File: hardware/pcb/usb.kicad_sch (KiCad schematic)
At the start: 6 parts, among them J3 USB_C_Receptacle_USB2.0_16P, U5 ECMF02-2AMX6

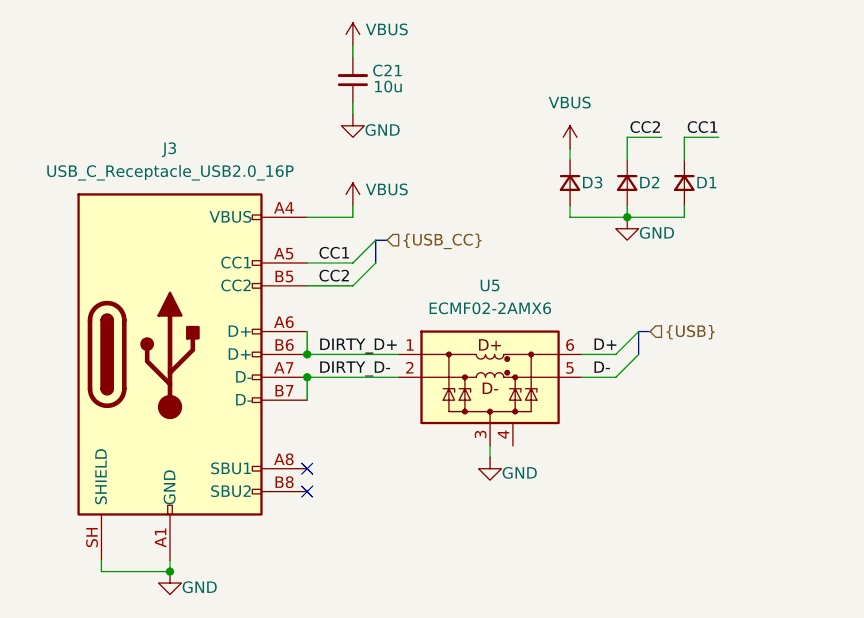
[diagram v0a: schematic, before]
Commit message: bunch of small changes
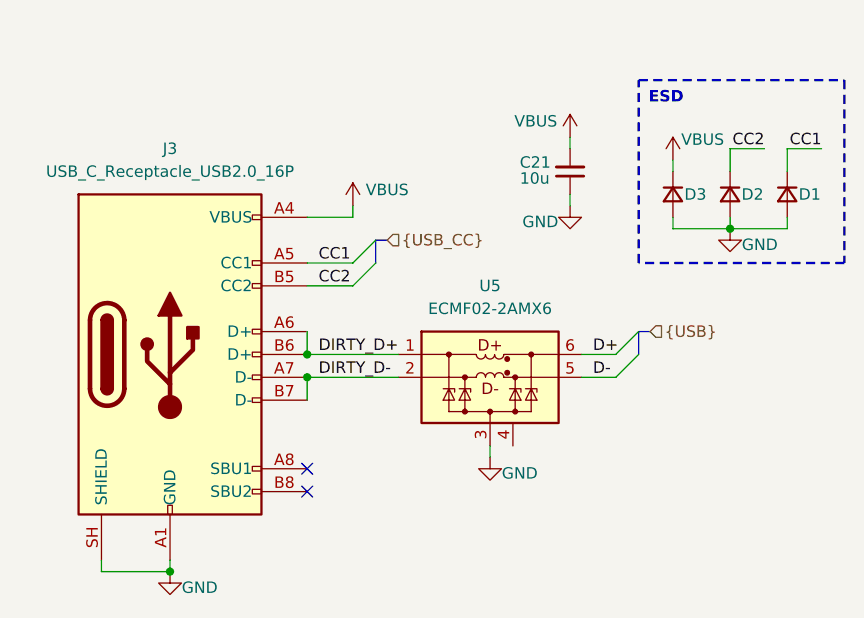
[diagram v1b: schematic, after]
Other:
- note added: "ESD"
- moved on the sheet: C21, D1, D2, D3

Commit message: bunch of small audio changes
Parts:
- J3: footprint (none) -> PCM_ckl-connector:USB_C_Receptacle_HRO_TYPE-C-31-M-12
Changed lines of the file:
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@@
 			)
 		)
-		(property "Footprint" ""
+		(property "Footprint" "PCM_ckl-connector:USB_C_Receptacle_HRO_TYPE-C-31-M-12"
 			(at 90.17 63.5 0)
 			(hide yes)
